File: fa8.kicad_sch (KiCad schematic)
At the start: 7 parts, among them U1 4081, U10 4071, U18 4069, U27 4069, U46 4071, U48 4081, U6 4081

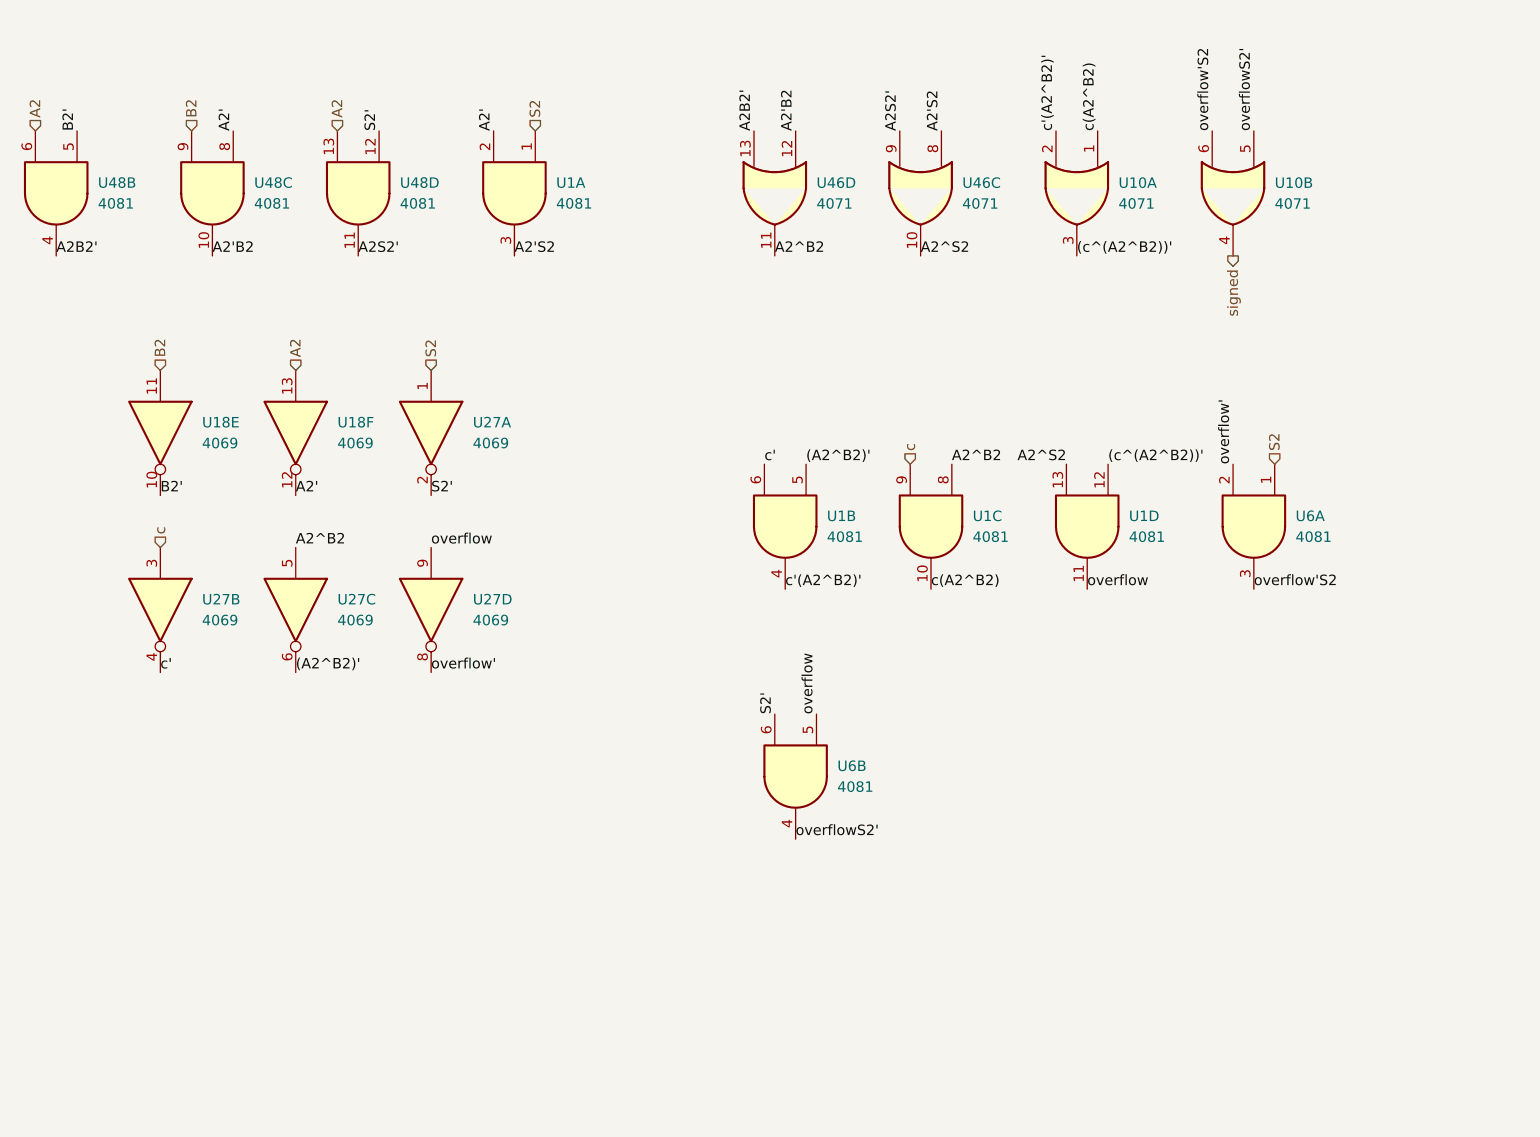
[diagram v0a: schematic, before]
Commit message: Add files via upload
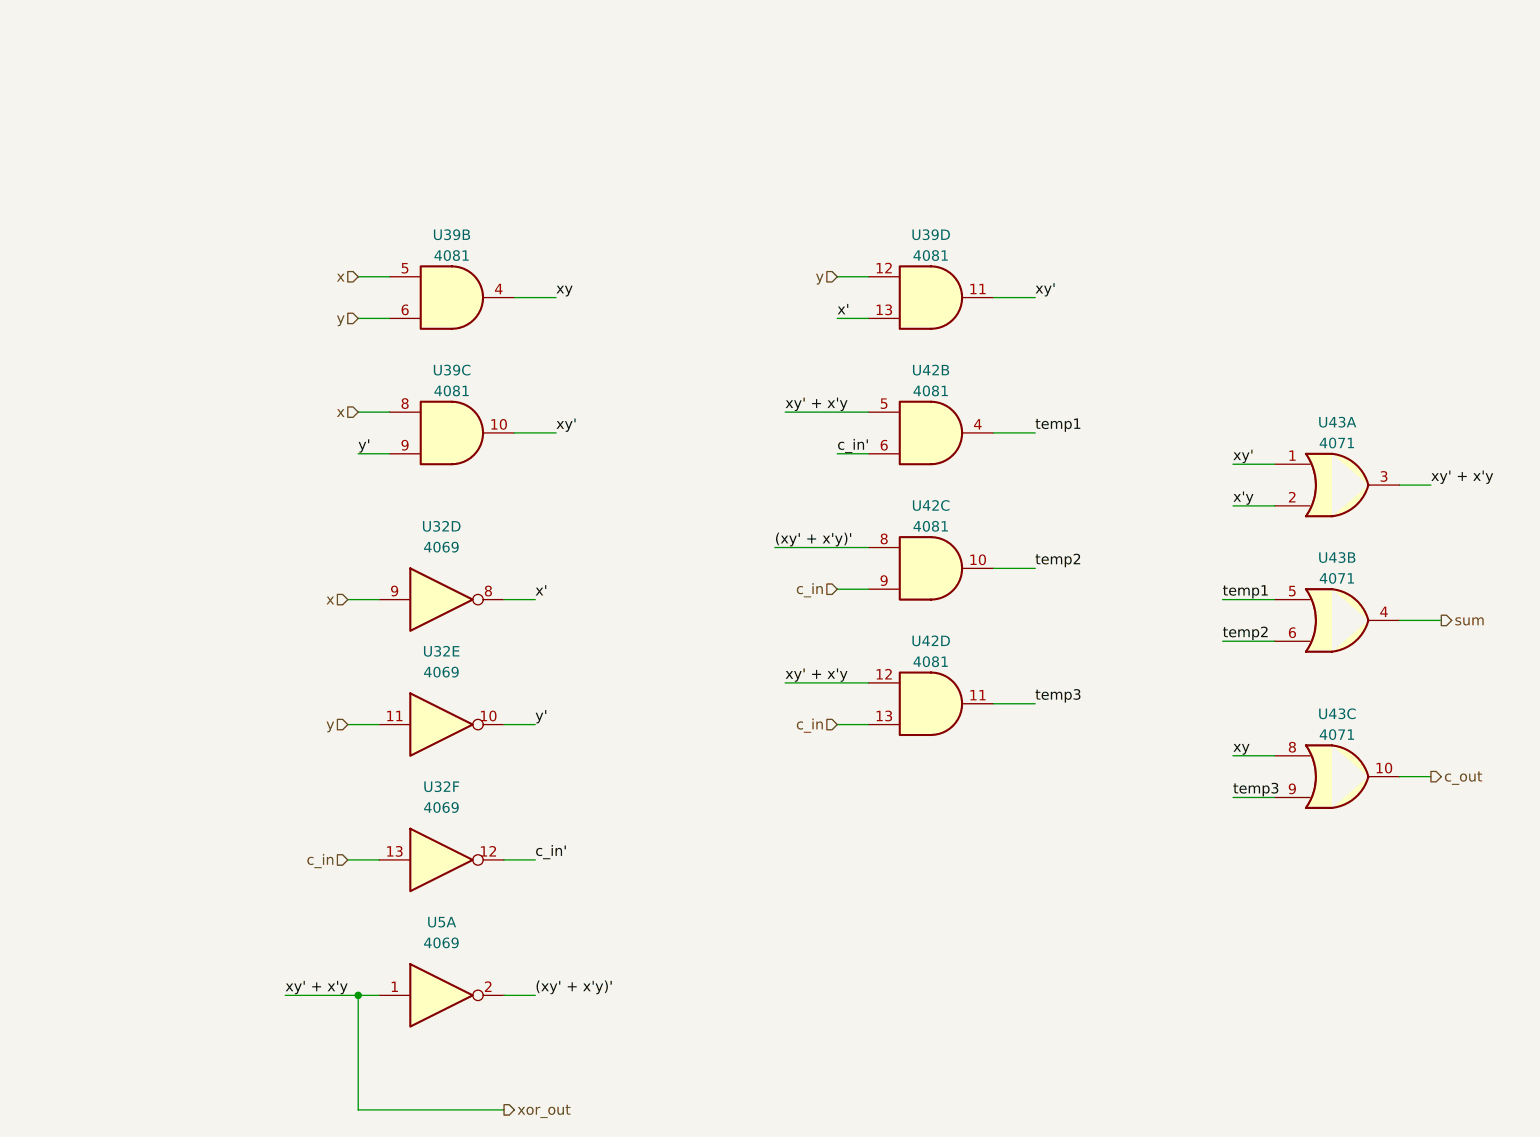
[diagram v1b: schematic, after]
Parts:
- removed U1, U48, U6: 4081, Package_DIP:CERDIP-14_W7.62mm_SideBrazed_LongPads_Socket, symbol 4xxx:4081
- removed U10, U46: 4071, Package_DIP:CERDIP-14_W7.62mm_SideBrazed_LongPads_Socket, symbol 4xxx:4071
- removed U18, U27: 4069, Package_DIP:CERDIP-14_W7.62mm_SideBrazed_LongPads_Socket, symbol 4xxx:4069
- added U32, U5: 4069, Package_DIP:CERDIP-14_W7.62mm_SideBrazed_LongPads_Socket, symbol 4xxx:4069
- added U39, U42: 4081, Package_DIP:CERDIP-14_W7.62mm_SideBrazed_LongPads_Socket, symbol 4xxx:4081
- added U43: 4071, Package_DIP:CERDIP-14_W7.62mm_SideBrazed_LongPads_Socket, symbol 4xxx:4071
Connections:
- new net (xy' + x'y)': U42.8, U5.2
- new net c_in: U32.13, U42.13, U42.9
- new net c_in': U32.12, U42.6
- new net c_out: U43.10
- new net sum: U43.4
- new net temp1: U42.4, U43.5
- new net temp2: U42.10, U43.6
- new net temp3: U42.11, U43.9
- new net x: U32.9, U39.5, U39.8
- new net x': U32.8, U39.13
- new net x'y: U43.2
- new net xor_out: U42.12, U42.5, U43.3, U5.1
- new net xy: U39.4, U43.8
- new net xy': U39.10, U39.11, U43.1
- new net y: U32.11, U39.12, U39.6
- new net y': U32.10, U39.9
